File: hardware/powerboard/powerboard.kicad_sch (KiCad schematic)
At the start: 66 parts, among them J1 USB_B_Micro, J10 5V Header, J11 3V3 Header, J2 Boot, J3 Power, J4 Display, J5 Debug, J6 SPI_1, J7 I2C_0, J8 I2C_1, J9 UART_0, SW1 Oct_Up, SW2 RESET, SW3 Oct_Down, SW4 RotaryEncoder_Switch, U2 MCP1603, U3 RP2040, U4 W25Q128JVSIM, Y1 Crystal_GND24

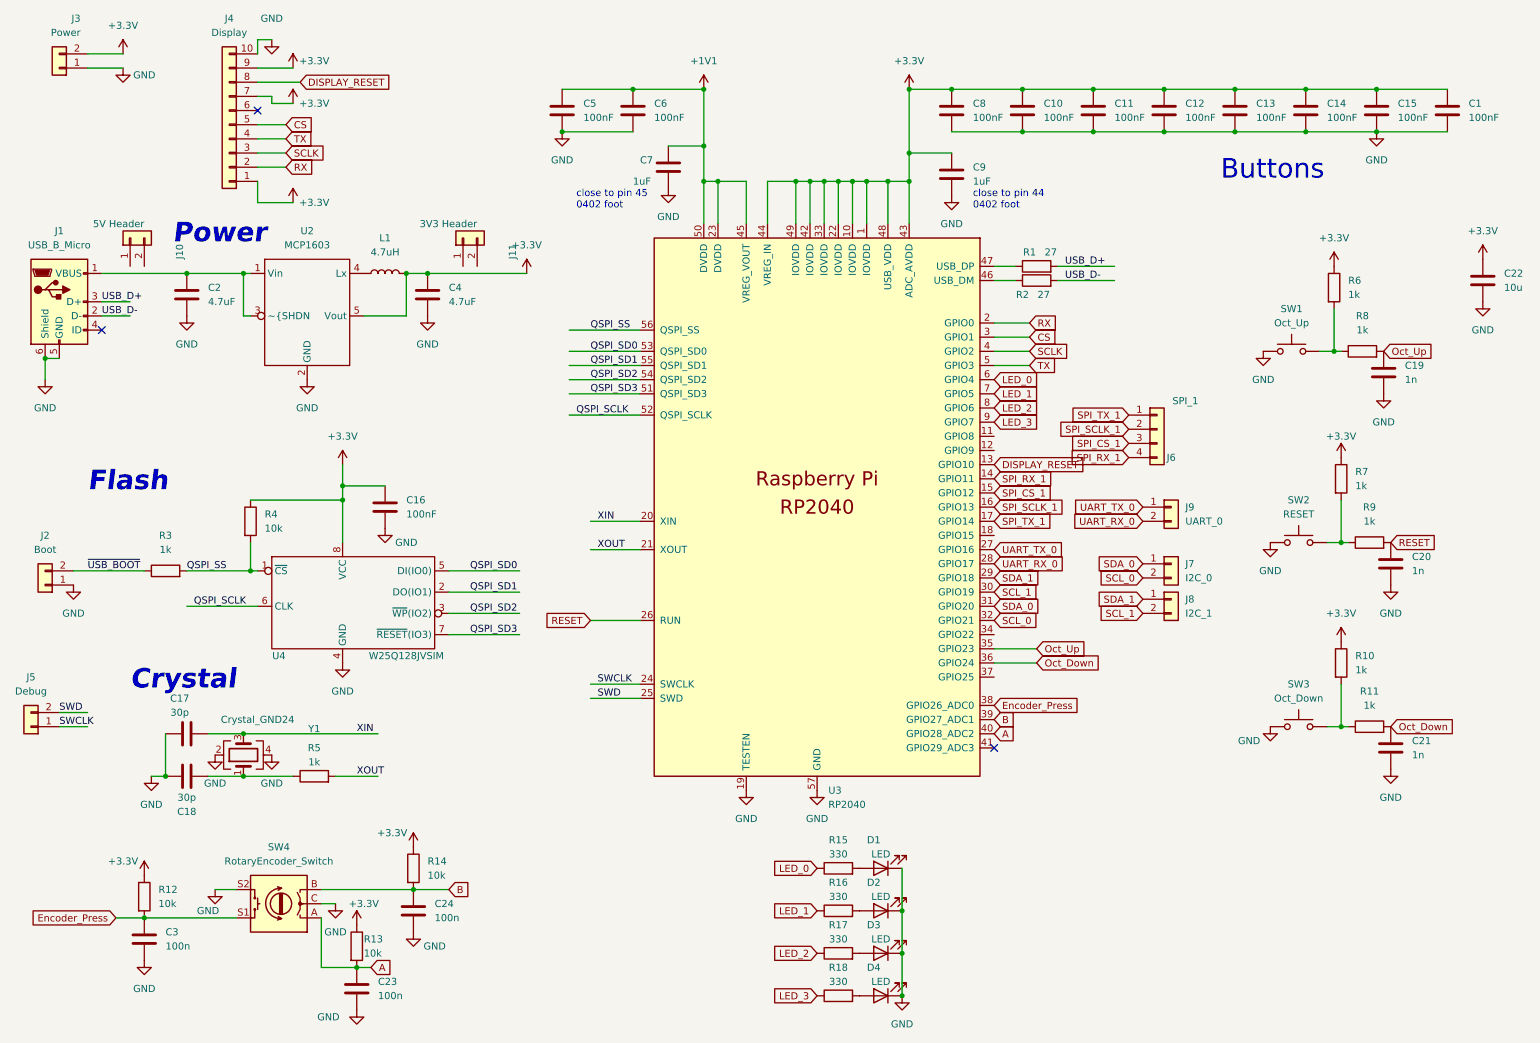
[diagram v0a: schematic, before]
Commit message: Powerboard review with sheaff
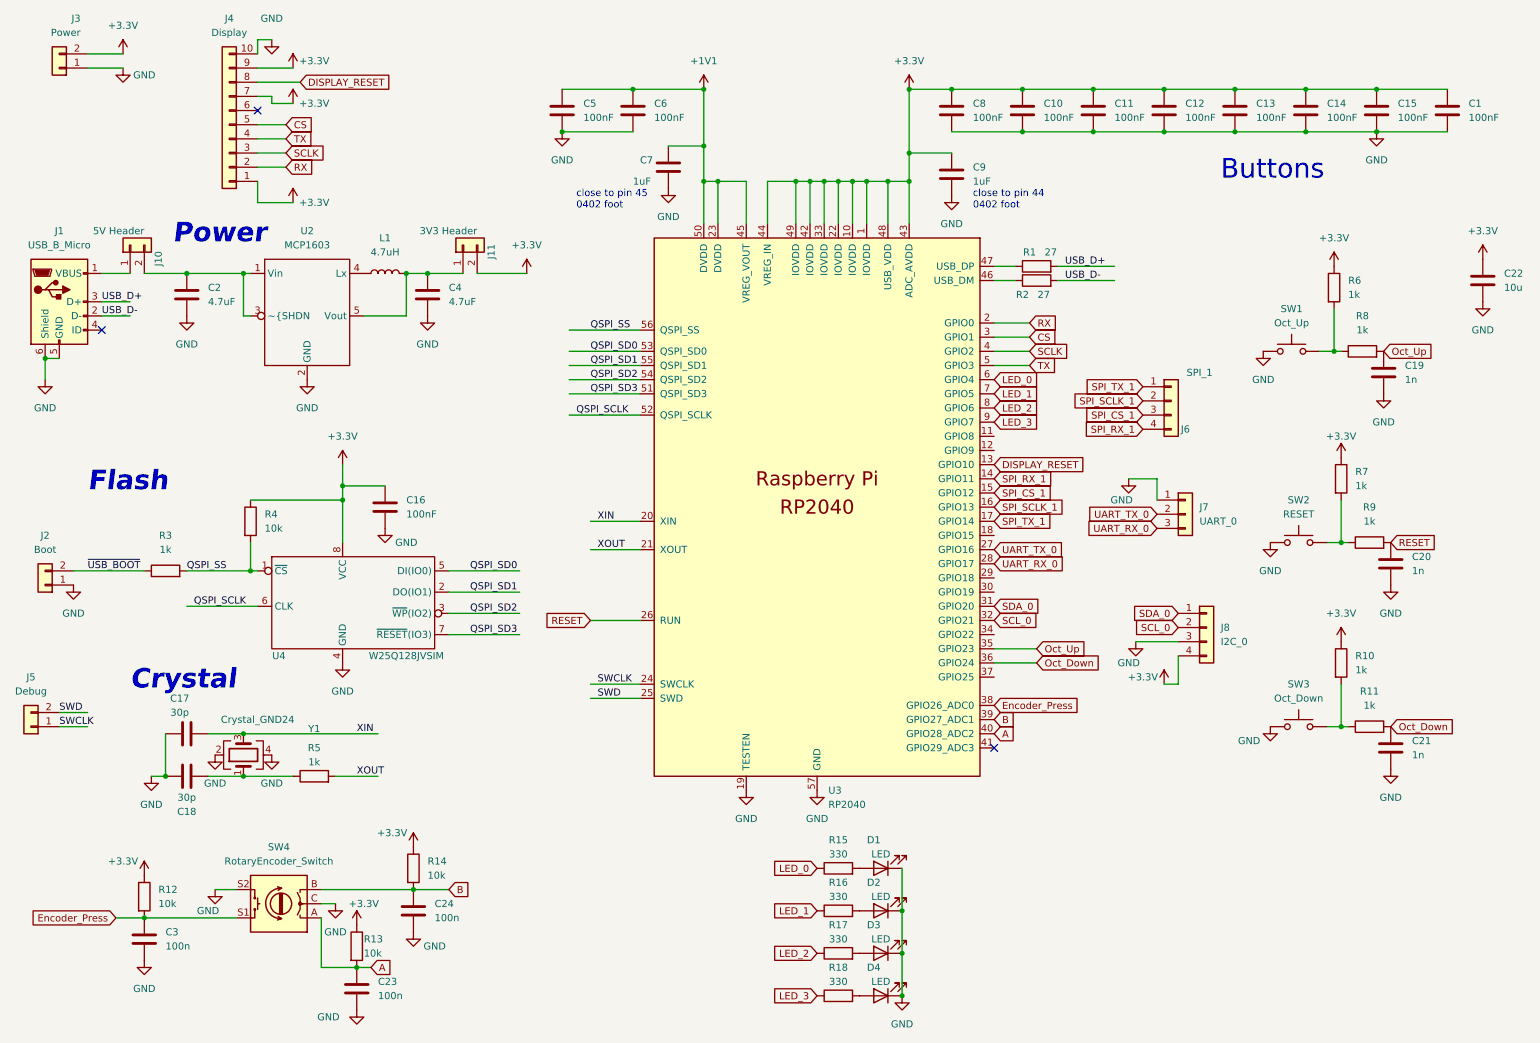
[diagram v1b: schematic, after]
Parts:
- removed J7: I2C_0, Connector_PinHeader_2.54mm:PinHeader_1x02_P2.54mm_Vertical, symbol Connector_Generic:Conn_01x02
- removed J8: I2C_1, Connector_PinHeader_2.54mm:PinHeader_1x02_P2.54mm_Vertical, symbol Connector_Generic:Conn_01x02
- removed J9: UART_0, Connector_PinHeader_2.54mm:PinHeader_1x02_P2.54mm_Vertical, symbol Connector_Generic:Conn_01x02
- added J7: UART_0, Connector_PinSocket_2.54mm:PinSocket_1x03_P2.54mm_Vertical, symbol Connector_Generic:Conn_01x03
- added J8: I2C_0, Connector_PinSocket_2.54mm:PinSocket_1x04_P2.54mm_Vertical, symbol Connector_Generic:Conn_01x04
- J10, J11: footprint Connector_PinHeader_2.54mm:PinHeader_1x02_P2.54mm_Horizontal -> Connector_PinHeader_2.54mm:PinHeader_1x02_P2.54mm_Vertical
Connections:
- net +3.3V: now also J11.2 (Pin_2), J8.4 (Pin_4); no longer C4.1, L1.2, U2.5 (Vout)
- net GND: now also J7.1 (Pin_1), J8.3 (Pin_3)
- net SCL_0: now also J8.2 (Pin_2)
- net SDA_0: now also J8.1 (Pin_1)
- net UART_RX_0: now also J7.3 (Pin_3)
- net UART_TX_0: now also J7.2 (Pin_2)
- net at C2.1, U2.1 (Vin), U2.3 (~{SHDN): now also J10.2 (Pin_2); no longer J1.1 (VBUS)
- net at J10.1 (Pin_1): now also J1.1 (VBUS)
- net at J11.1 (Pin_1): now also C4.1, L1.2, U2.5 (Vout)
- net SCL_1: no longer names the net of U3.30 (GPIO19)
- net SDA_1: no longer names the net of U3.29 (GPIO18)
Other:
- moved on the sheet: J10, J11, J6
